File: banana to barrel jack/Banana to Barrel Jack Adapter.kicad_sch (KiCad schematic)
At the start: 10 parts, among them J1 Barrel_Jack_Switch, J2 Positive, J3 Negative

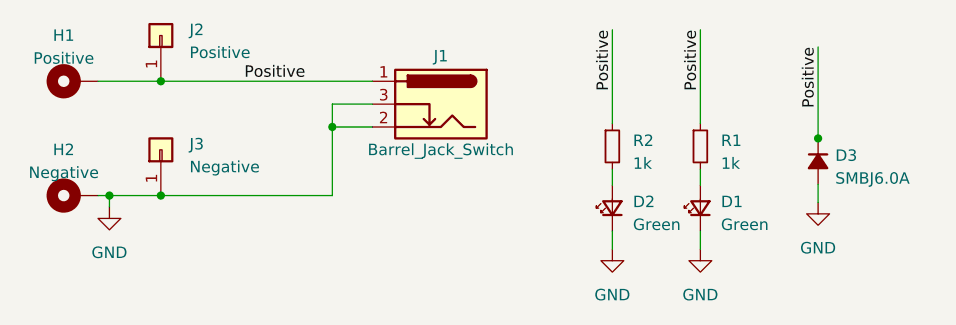
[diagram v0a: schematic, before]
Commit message: Cleared DRC issues
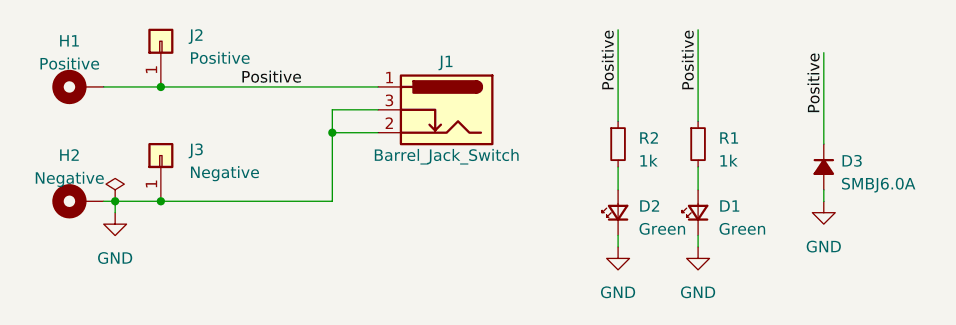
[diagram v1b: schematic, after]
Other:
- moved on the sheet: D1, D2, D3, H1, H2, J1, J2, J3, R2
